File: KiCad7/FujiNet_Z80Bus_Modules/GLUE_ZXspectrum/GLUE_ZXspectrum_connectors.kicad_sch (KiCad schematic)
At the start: 2 parts, among them J1 Conn_02x12_Odd_Even, J2 Conn_02x12_Odd_Even

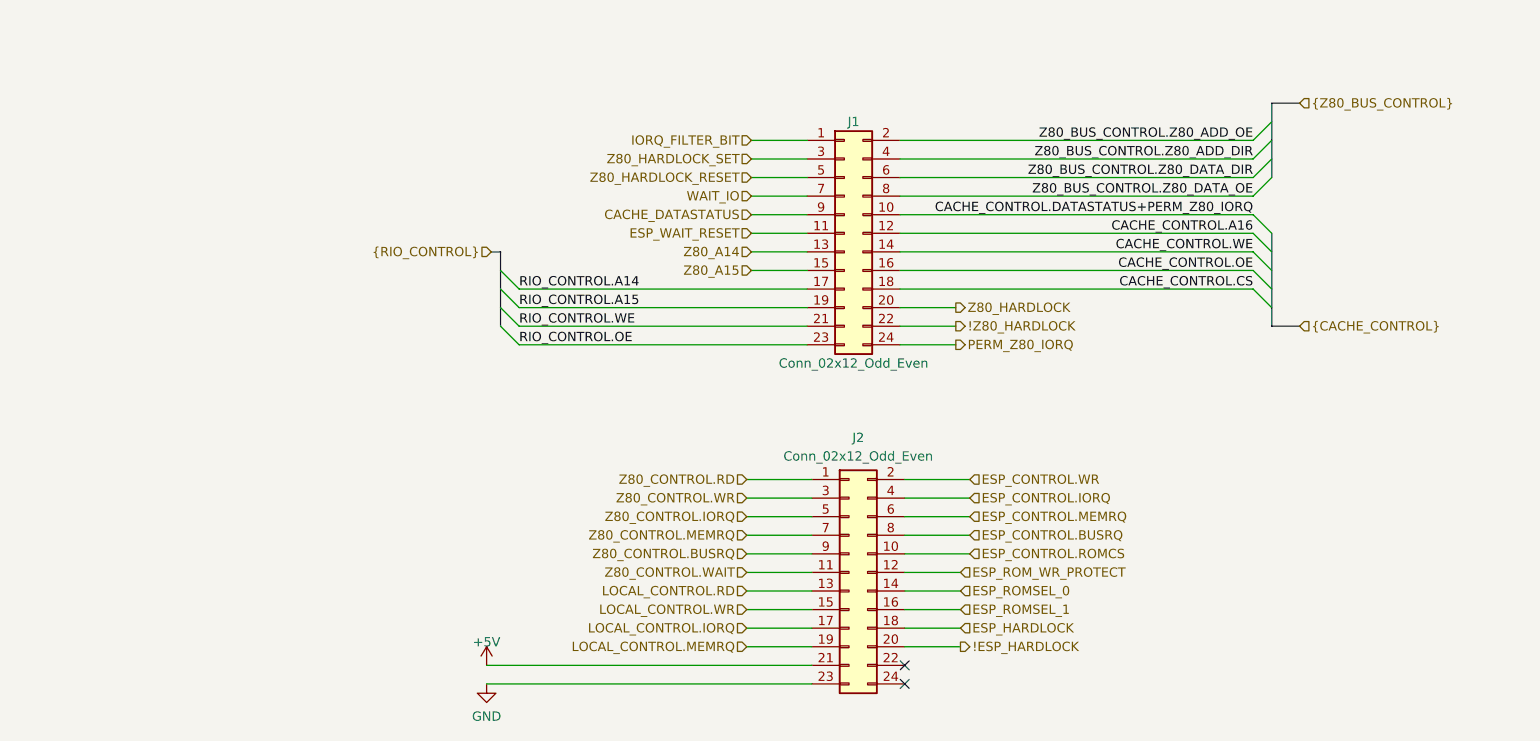
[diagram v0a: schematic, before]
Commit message: KiCad FIXED GLUE
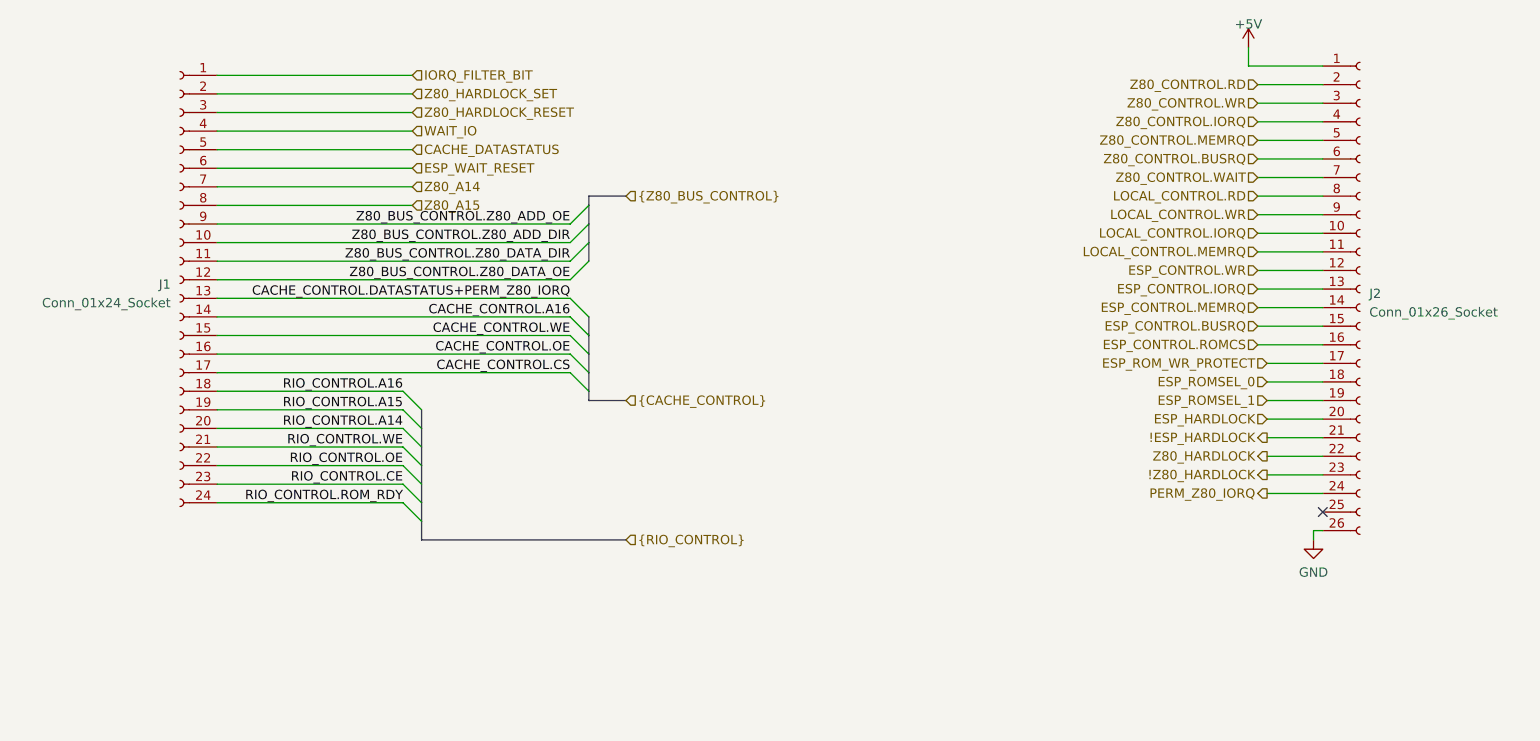
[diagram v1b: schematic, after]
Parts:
- removed J1, J2: Conn_02x12_Odd_Even, Connector_PinHeader_2.54mm:PinHeader_2x16_P2.54mm_Vertical, symbol Connector_Generic:Conn_02x12_Odd_Even
- added J1: Conn_01x24_Socket, Connector_PinSocket_2.54mm:PinSocket_1x24_P2.54mm_Vertical, symbol Connector:Conn_01x24_Socket
- added J2: Conn_01x26_Socket, Connector_PinSocket_2.54mm:PinSocket_1x26_P2.54mm_Vertical, symbol Connector:Conn_01x26_Socket
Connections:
- net !ESP_HARDLOCK: now also J2.21 (Pin_21)
- net !Z80_HARDLOCK: now also J2.23 (Pin_23)
- net +5V: now also J2.1 (Pin_1)
- net CACHE_CONTROL.A16: now also J1.14 (Pin_14)
- net CACHE_CONTROL.CS: now also J1.17 (Pin_17)
- net CACHE_CONTROL.DATASTATUS+PERM_Z80_IORQ: now also J1.13 (Pin_13)
- net CACHE_CONTROL.OE: now also J1.16 (Pin_16)
- net CACHE_CONTROL.WE: now also J1.15 (Pin_15)
- net CACHE_DATASTATUS: now also J1.5 (Pin_5)
- net ESP_CONTROL.BUSRQ: now also J2.15 (Pin_15)
- net ESP_CONTROL.IORQ: now also J2.13 (Pin_13)
- net ESP_CONTROL.MEMRQ: now also J2.14 (Pin_14)
- net ESP_CONTROL.ROMCS: now also J2.16 (Pin_16)
- net ESP_CONTROL.WR: now also J2.12 (Pin_12)
- net ESP_HARDLOCK: now also J2.20 (Pin_20)
- net ESP_ROMSEL_0: now also J2.18 (Pin_18)
- net ESP_ROMSEL_1: now also J2.19 (Pin_19)
- net ESP_ROM_WR_PROTECT: now also J2.17 (Pin_17)
- net ESP_WAIT_RESET: now also J1.6 (Pin_6)
- net GND: now also J2.26 (Pin_26)
- net IORQ_FILTER_BIT: now also J1.1 (Pin_1)
- net LOCAL_CONTROL.IORQ: now also J2.10 (Pin_10)
- net LOCAL_CONTROL.MEMRQ: now also J2.11 (Pin_11)
- net LOCAL_CONTROL.RD: now also J2.8 (Pin_8)
- net LOCAL_CONTROL.WR: now also J2.9 (Pin_9)
- net PERM_Z80_IORQ: now also J2.24 (Pin_24)
- net RIO_CONTROL.A14: now also J1.20 (Pin_20)
- net RIO_CONTROL.A15: now also J1.19 (Pin_19)
- net RIO_CONTROL.OE: now also J1.22 (Pin_22)
- net RIO_CONTROL.WE: now also J1.21 (Pin_21)
- net WAIT_IO: now also J1.4 (Pin_4)
- net Z80_A14: now also J1.7 (Pin_7)
- net Z80_A15: now also J1.8 (Pin_8)
- net Z80_BUS_CONTROL.Z80_ADD_DIR: now also J1.10 (Pin_10)
- net Z80_BUS_CONTROL.Z80_ADD_OE: now also J1.9 (Pin_9)
- net Z80_BUS_CONTROL.Z80_DATA_DIR: now also J1.11 (Pin_11)
- net Z80_BUS_CONTROL.Z80_DATA_OE: now also J1.12 (Pin_12)
- net Z80_CONTROL.BUSRQ: now also J2.6 (Pin_6)
- net Z80_CONTROL.IORQ: now also J2.4 (Pin_4)
- net Z80_CONTROL.MEMRQ: now also J2.5 (Pin_5)
- net Z80_CONTROL.RD: now also J2.2 (Pin_2)
- net Z80_CONTROL.WAIT: now also J2.7 (Pin_7)
- net Z80_CONTROL.WR: now also J2.3 (Pin_3)
- net Z80_HARDLOCK: now also J2.22 (Pin_22)
- net Z80_HARDLOCK_RESET: now also J1.3 (Pin_3)
- net Z80_HARDLOCK_SET: now also J1.2 (Pin_2)
- new net RIO_CONTROL.A16: J1.18 (Pin_18)
- new net RIO_CONTROL.CE: J1.23 (Pin_23)
- new net RIO_CONTROL.ROM_RDY: J1.24 (Pin_24)
- no-connect marks 2 -> 1
